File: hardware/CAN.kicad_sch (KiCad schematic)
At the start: 5 parts, among them U1 MCP2542FDxMF

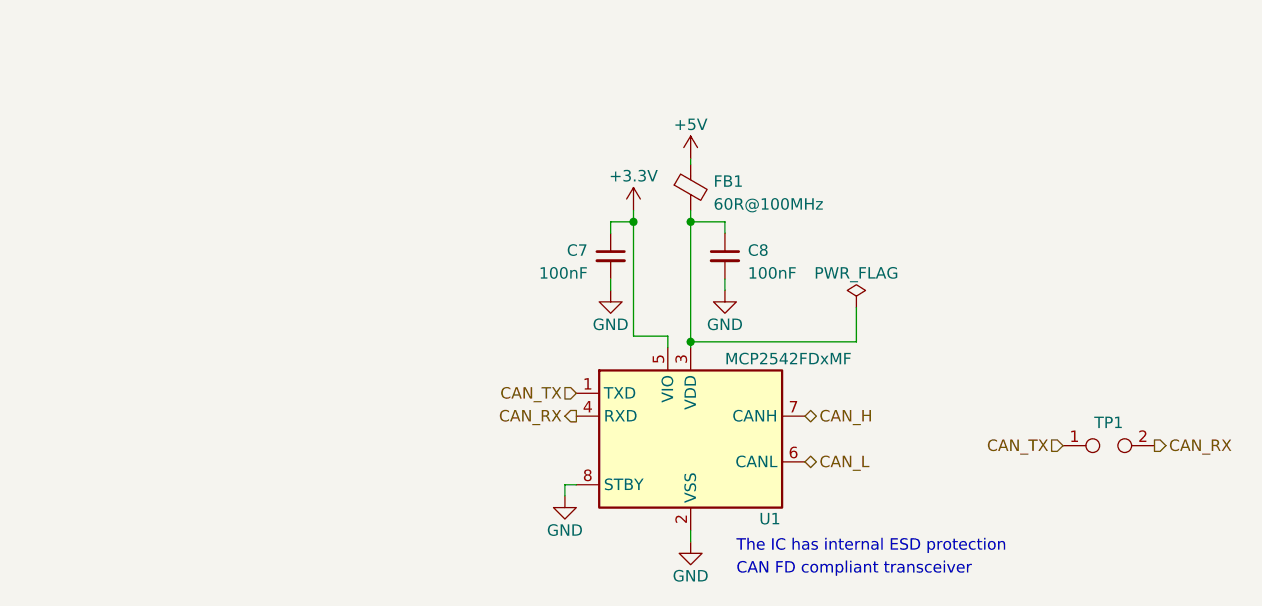
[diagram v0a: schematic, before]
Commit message: Placement done
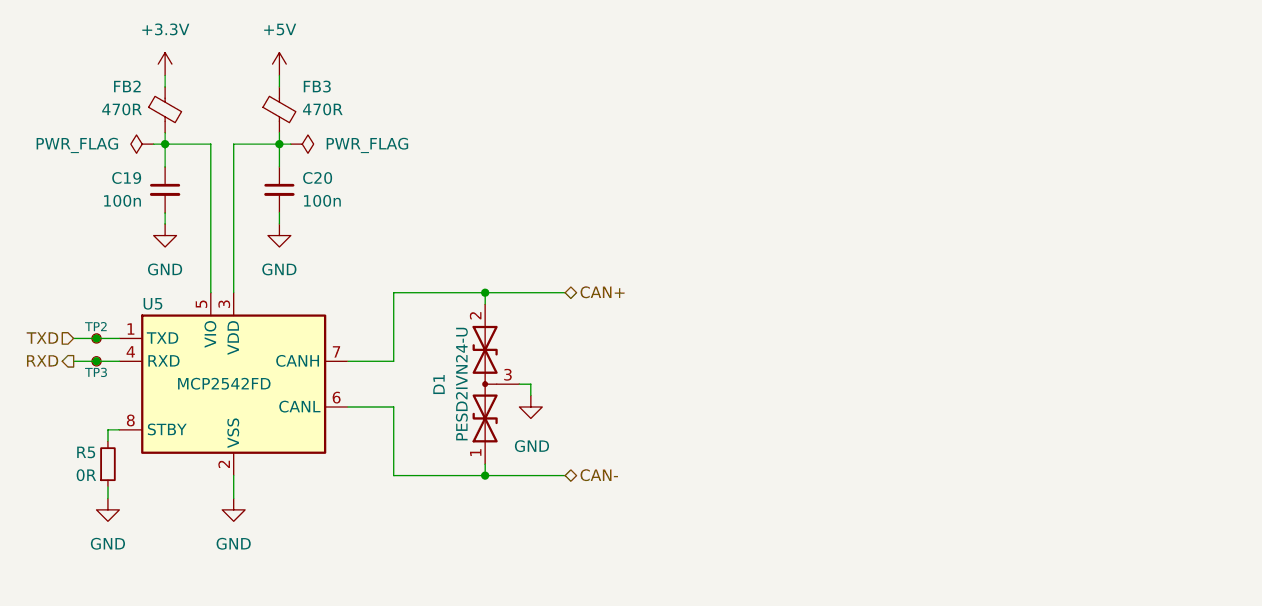
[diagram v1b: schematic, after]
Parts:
- removed C7, C8: 100nF, Capacitor_SMD:C_0603_1608Metric, symbol Device:C_Small
- removed FB1: 60R@100MHz, Inductor_SMD:L_0603_1608Metric, symbol Device:FerriteBead_Small
- removed TP1: TestPoint_2Pole, TestPoint:TestPoint_2Pads_Pitch2.54mm_Drill0.8mm, symbol Connector:TestPoint_2Pole
- removed U1: MCP2542FDxMF, Package_DFN_QFN:DFN-8-1EP_3x3mm_P0.65mm_EP1.55x2.4mm, symbol Interface_CAN_LIN:MCP2542FDxMF
- added C19, C20: 100n, Capacitor_SMD:C_0603_1608Metric, symbol Device:C_Small
- added D1: PESD2IVN24-U, Package_TO_SOT_SMD:SOT-323_SC-70, symbol Device:D_TVS_Dual_AAC
- added FB2, FB3: 470R, Inductor_SMD:L_0603_1608Metric, symbol Device:FerriteBead_Small
- added R5: 0R, Resistor_SMD:R_0603_1608Metric, symbol Device:R_Small
- added TP2, TP3: TestPoint_Small, TestPoint:TestPoint_Pad_D1.0mm, symbol Connector:TestPoint_Small
- added U5: MCP2542FD, Package_DFN_QFN:DFN-8-1EP_3x3mm_P0.65mm_EP1.55x2.4mm, symbol Interface_CAN_LIN:MCP2542FDxMF
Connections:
- net +3.3V: now also FB2.1
- net +5V: now also FB3.1
- net GND: now also C19.2, C20.2, D1.3 (common), R5.1, U5.2 (VSS), U5.9 (VSS)
- new net: C20.1, FB3.2, U5.3 (VDD)
- new net: C19.1, FB2.2, U5.5 (VIO)
- new net: R5.2, U5.8 (STBY)
- new net CAN+: D1.2 (A2), U5.7 (CANH)
- new net CAN-: D1.1 (A1), U5.6 (CANL)
- new net RXD: TP3.1, U5.4 (RXD)
- new net TXD: TP2.1, U5.1 (TXD)
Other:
- note removed: "CAN FD compliant transceiver"
- note removed: "The IC has internal ESD protection"

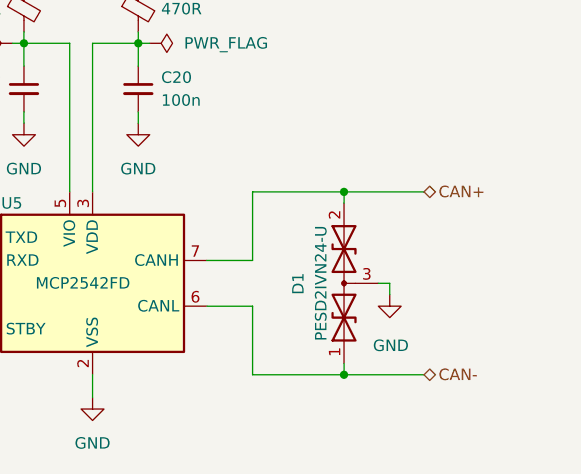
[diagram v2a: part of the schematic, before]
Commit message: Fix minor issues
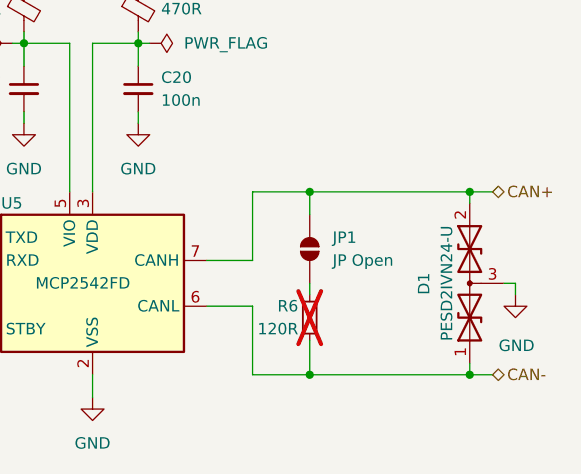
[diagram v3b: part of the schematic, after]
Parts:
- added JP1: JP Open, Jumper:SolderJumper-2_P1.3mm_Open_Pad1.0x1.5mm, symbol Jumper:SolderJumper_2_Open
- added R6: 120R, Resistor_SMD:R_0603_1608Metric, symbol Device:R_Small
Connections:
- net CAN+: now also JP1.2 (B)
- net CAN-: now also R6.1
- new net: JP1.1 (A), R6.2
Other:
- moved on the sheet: D1
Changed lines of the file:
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@@
+	)
+	(junction
+		(at 163.83 115.57)
+		(diameter 0)
+		(color 0 0 0 0)
 	)
 	(junction
@@
 	)
 	(junction
-		(at 167.64 115.57)
+		(at 181.61 115.57)
 		(diameter 0)
 		(color 0 0 0 0)
 	)
 	(junction
-		(at 167.64 95.25)
+		(at 181.61 95.25)
 		(diameter 0)
 		(color 0 0 0 0)
 	)
+	(junction
+		(at 163.83 95.25)
+		(diameter 0)
+		(color 0 0 0 0)
+	)
 	(wire
 		(pts
@@
 	(wire
 		(pts
+			(xy 163.83 95.25) (xy 181.61 95.25)
+		)
+		(stroke
+			(width 0)
+			(type default)
+		)
+	)
+	(wire
+		(pts
 			(xy 125.73 118.11) (xy 125.73 116.84)
 		)
@@
 	(wire
 		(pts
+			(xy 181.61 115.57) (xy 184.15 115.57)
+		)
+		(stroke
+			(width 0)
+			(type default)
+		)
+	)
+	(wire
+		(pts
+			(xy 163.83 105.41) (xy 163.83 106.68)
+		)
+		(stroke
+			(width 0)
+			(type default)
+		)
+	)
+	(wire
+		(pts
+			(xy 181.61 95.25) (xy 184.15 95.25)
+		)
+		(stroke
+			(width 0)
+			(type default)
+		)
+	)
+	(wire
+		(pts
 			(xy 139.7 115.57) (xy 139.7 118.11)
 		)
@@
 	(wire
 		(pts
-			(xy 167.64 114.3) (xy 167.64 115.57)
+			(xy 181.61 114.3) (xy 181.61 115.57)
+		)
+		(stroke
+			(width 0)
+			(type default)
+		)
+	)
+	(wire
+		(pts
+			(xy 163.83 111.76) (xy 163.83 115.57)
 		)
 		(stroke
@@
 	(wire
 		(pts
-			(xy 172.72 106.68) (xy 172.72 105.41)
-		)
-		(stroke
-			(width 0)
-			(type default)
-		)
-	)
-	(wire
-		(pts
-			(xy 167.64 95.25) (xy 176.53 95.25)
+			(xy 186.69 106.68) (xy 186.69 105.41)
 		)
 		(stroke
@@
 	(wire
 		(pts
-			(xy 157.48 95.25) (xy 167.64 95.25)
+			(xy 157.48 95.25) (xy 163.83 95.25)
 		)
 		(stroke
@@
 	(wire
 		(pts
+			(xy 163.83 115.57) (xy 181.61 115.57)
+		)
+		(stroke
+			(width 0)
+			(type default)
+		)
+	)
+	(wire
+		(pts
 			(xy 124.46 100.33) (xy 127 100.33)
 		)
@@
 	(wire
 		(pts
-			(xy 167.64 115.57) (xy 176.53 115.57)
-		)
-		(stroke
-			(width 0)
-			(type default)
-		)
-	)
-	(wire
-		(pts
-			(xy 171.45 105.41) (xy 172.72 105.41)
+			(xy 185.42 105.41) (xy 186.69 105.41)
 		)
 		(stroke
@@
 	(wire
 		(pts
+			(xy 163.83 97.79) (xy 163.83 95.25)
+		)
+		(stroke
+			(width 0)
+			(type default)
+		)
+	)
+	(wire
+		(pts
 			(xy 157.48 107.95) (xy 157.48 115.57)
 		)
@@
 	(wire
 		(pts
-			(xy 167.64 95.25) (xy 167.64 96.52)
+			(xy 181.61 95.25) (xy 181.61 96.52)
 		)
 		(stroke
@@
 	(wire
 		(pts
-			(xy 157.48 115.57) (xy 167.64 115.57)
+			(xy 157.48 115.57) (xy 163.83 115.57)
 		)
 		(stroke
@@
 	(hierarchical_label "CAN-"
 		(shape bidirectional)
-		(at 176.53 115.57 0)
+		(at 184.15 115.57 0)
 		(fields_autoplaced yes)
 		(effects
@@
 	(hierarchical_label "CAN+"
 		(shape bidirectional)
-		(at 176.53 95.25 0)
+		(at 184.15 95.25 0)
 		(fields_autoplaced yes)
 		(effects
@@
 	(symbol
 		(lib_id "Device:D_TVS_Dual_AAC")
-		(at 167.64 105.41 90)
+		(at 181.61 105.41 90)
 		(unit 1)
 		(exclude_from_sim no)
@@
 		(dnp no)
 		(property "Reference" "D1"
-			(at 162.56 106.68 0)
+			(at 176.53 106.68 0)
 			(effects
 				(font
@@
 		)
 		(property "Value" "PESD2IVN24-U"
-			(at 165.1 105.41 0)
+			(at 179.07 105.41 0)
 			(effects
 				(font
@@
 		)
 		(property "Footprint" "Package_TO_SOT_SMD:SOT-323_SC-70"
-			(at 167.64 109.22 0)
+			(at 181.61 109.22 0)
 			(effects
 				(font
@@
 		)
 		(property "Datasheet" "~"
-			(at 167.64 109.22 0)
-			(effects
-				(font
-					(size 1.27 1.27)
-				)
-				(hide yes)
-			)
-		)
-		(property "Description" ""
-			(at 167.64 105.41 0)
+			(at 181.61 109.22 0)
+			(effects
+				(font
+					(size 1.27 1.27)
+				)
+				(hide yes)
+			)
+		)
+		(property "Description" ""
+			(at 181.61 105.41 0)
 			(effects
 				(font
@@
 	)
 	(symbol
+		(lib_id "Jumper:SolderJumper_2_Open")
+		(at 163.83 101.6 90)
+		(unit 1)
+		(exclude_from_sim yes)
+		(in_bom no)
+		(on_board yes)
+		(dnp no)
+		(fields_autoplaced yes)
+		(property "Reference" "JP1"
+			(at 166.37 100.3299 90)
+			(effects
+				(font
+					(size 1.27 1.27)
+				)
+				(justify right)
+			)
+		)
+		(property "Value" "JP Open"
+			(at 166.37 102.8699 90)
+			(effects
+				(font
+					(size 1.27 1.27)
+				)
+				(justify right)
+			)
+		)
+		(property "Footprint" "Jumper:SolderJumper-2_P1.3mm_Open_Pad1.0x1.5mm"
+			(at 163.83 101.6 0)
+			(effects
+				(font
+					(size 1.27 1.27)
+				)
+				(hide yes)
+			)
+		)
+		(property "Datasheet" "~"
+			(at 163.83 101.6 0)
+			(effects
+				(font
+					(size 1.27 1.27)
+				)
+				(hide yes)
+			)
+		)
+		(property "Description" "Solder Jumper, 2-pole, open"
+			(at 163.83 101.6 0)
+			(effects
+				(font
+					(size 1.27 1.27)
+				)
+				(hide yes)
+			)
+		)
+		(pin "1"
+		)
+		(pin "2"
+		)
+		(instances
+			(project "SteeringWheel"
+				(path "/b652b05a-4e3d-4ad1-b032-18886abe7d45/18d28e7d-3445-4022-b832-1432f129198e"
+					(reference "JP1")
+					(unit 1)
+				)
+			)
+		)
+	)
+	(symbol
 		(lib_id "power:GND")
 		(at 144.78 87.63 0)
@@
 	(symbol
 		(lib_id "power:GND")
-		(at 172.72 106.68 0)
+		(at 186.69 106.68 0)
 		(unit 1)
 		(exclude_from_sim no)
@@
 		(dnp no)
 		(property "Reference" "#U01"
-			(at 172.72 113.03 0)
+			(at 186.69 113.03 0)
 			(effects
 				(font
@@
 		)
 		(property "Value" "GND"
-			(at 172.847 112.3442 0)
+			(at 186.817 112.3442 0)
 			(effects
 				(font
@@
 		)
 		(property "Footprint" ""
-			(at 172.72 106.68 0)
+			(at 186.69 106.68 0)
 			(effects
 				(font
@@
 		)
 		(property "Datasheet" ""
-			(at 172.72 106.68 0)
-			(effects
-				(font
-					(size 1.27 1.27)
-				)
-				(hide yes)
-			)
-		)
-		(property "Description" ""
-			(at 172.72 106.68 0)
+			(at 186.69 106.68 0)
+			(effects
+				(font
+					(size 1.27 1.27)
+				)
+				(hide yes)
+			)
+		)
+		(property "Description" ""
+			(at 186.69 106.68 0)
 			(effects
 				(font
@@
 					(unit 1)
 				)
+			)
+		)
+	)
+	(symbol
+		(lib_id "Device:R_Small")
+		(at 163.83 109.22 0)
+		(mirror x)
+		(unit 1)
+		(exclude_from_sim no)
+		(in_bom yes)
+		(on_board yes)
+		(dnp yes)
+		(property "Reference" "R6"
+			(at 162.56 107.95 0)
+			(effects
+				(font
+					(size 1.27 1.27)
+				)
+				(justify right)
+			)
+		)
+		(property "Value" "120R"
+			(at 162.56 110.49 0)
+			(effects
+				(font
+					(size 1.27 1.27)
+				)
+				(justify right)
+			)
+		)
+		(property "Footprint" "Resistor_SMD:R_0603_1608Metric"
+			(at 163.83 109.22 0)
+			(effects
+				(font
+					(size 1.27 1.27)
+				)
+				(hide yes)
+			)
+		)
+		(property "Datasheet" "~"
+			(at 163.83 109.22 0)
+			(effects
+				(font
+					(size 1.27 1.27)
+				)
+				(hide yes)
+			)
+		)
+		(property "Description" ""
+			(at 163.83 109.22 0)
+			(effects
+				(font
+					(size 1.27 1.27)
+				)
+				(hide yes)
+			)
+		)
+		(pin "1"
+		)
+		(pin "2"
+		)
+		(instances
+			(project "SteeringWheel"
+				(path "/b652b05a-4e3d-4ad1-b032-18886abe7d45/18d28e7d-3445-4022-b832-1432f129198e"
+					(reference "R6")
+					(unit 1)
+				)
